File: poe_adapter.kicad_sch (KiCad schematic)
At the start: 7 parts

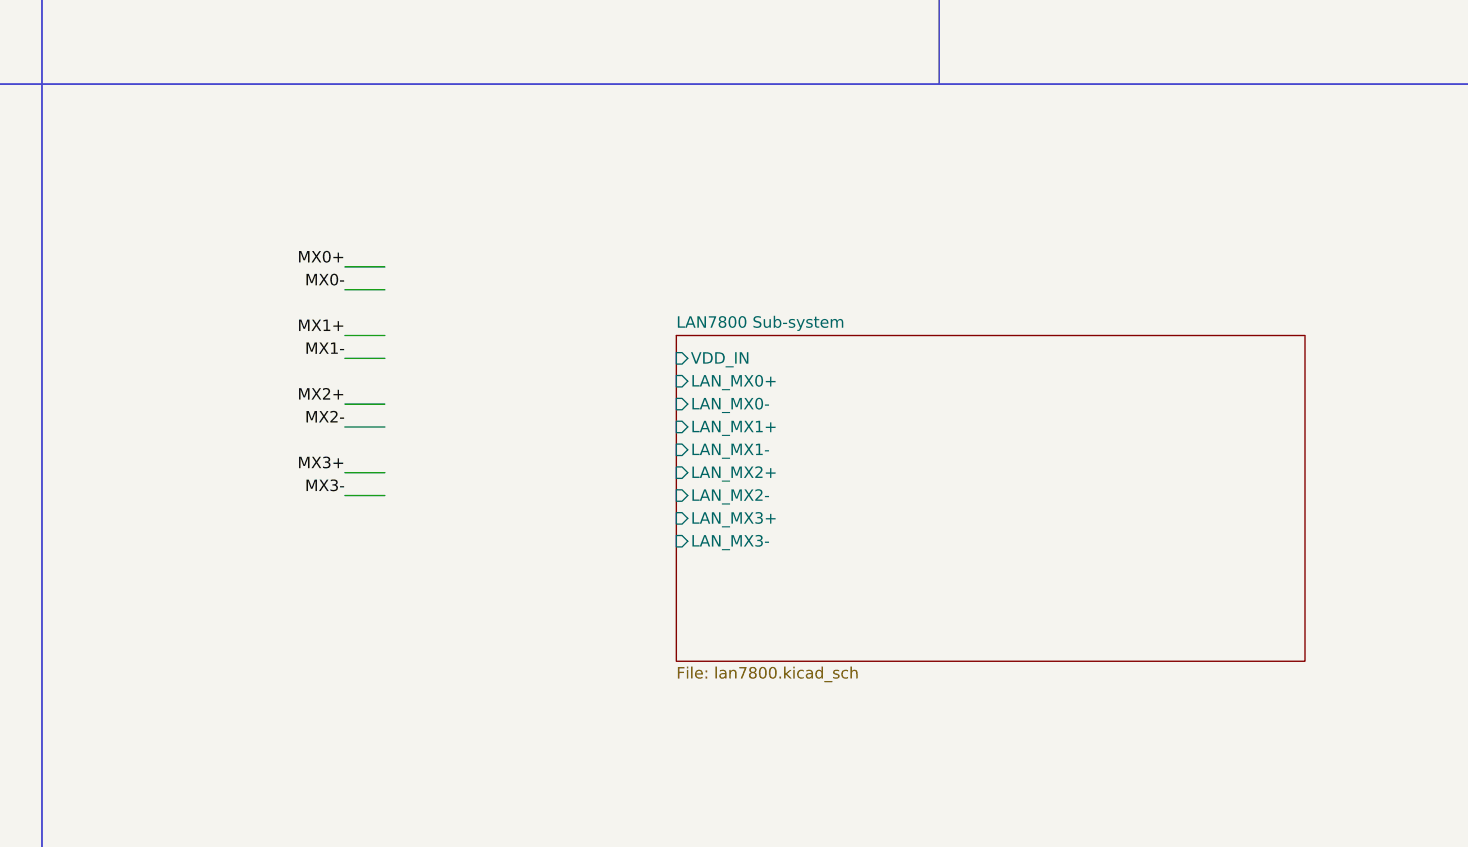
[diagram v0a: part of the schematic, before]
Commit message: LAN7800 Update 220707-2
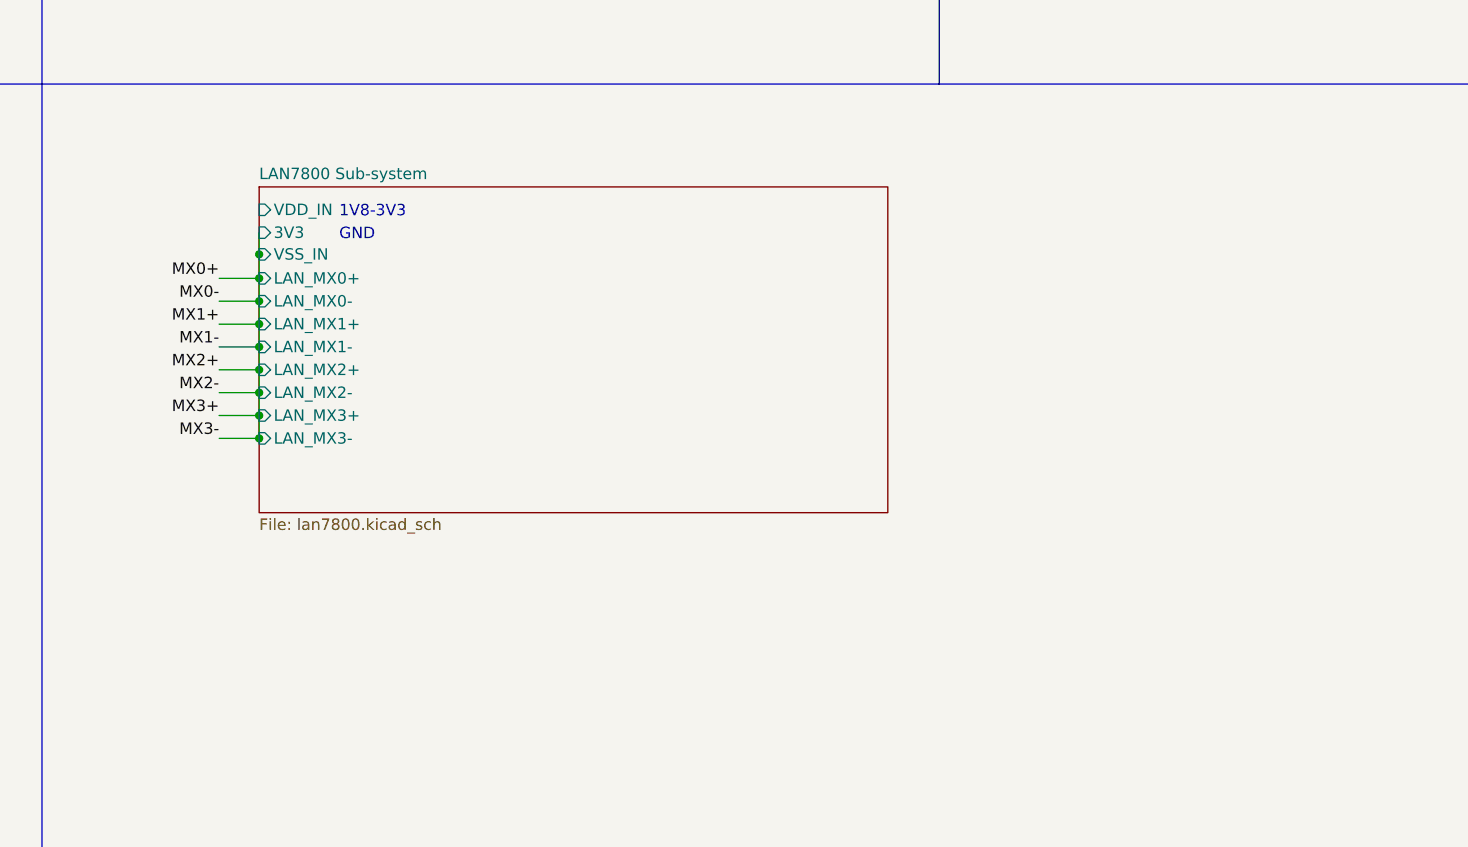
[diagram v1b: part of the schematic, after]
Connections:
- net MX0- is gone; now on net MX0+: TR?.11 (TD4+)
- net MX1+ is gone; now on net MX0+: TR?.9 (TD3-)
- net MX1- is gone; now on net MX0+: TR?.8 (TD3+)
- net MX2+ is gone; now on net MX0+: TR?.6 (TD2-)
- net MX2- is gone; now on net MX0+: TR?.5 (TD2+)
- net MX3+ is gone; now on net MX0+: TR?.3 (TD1-)
- net MX3- is gone; now on net MX0+: TR?.2 (TD1+)
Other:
- sheet LAN7800 Sub-system ports: added 3V3, VSS_IN; removed none
- note added: "1V8-3V3"
- note added: "GND"
